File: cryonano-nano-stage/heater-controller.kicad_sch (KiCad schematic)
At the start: 13 parts, among them U3 1ED3141MU12FXUMA1

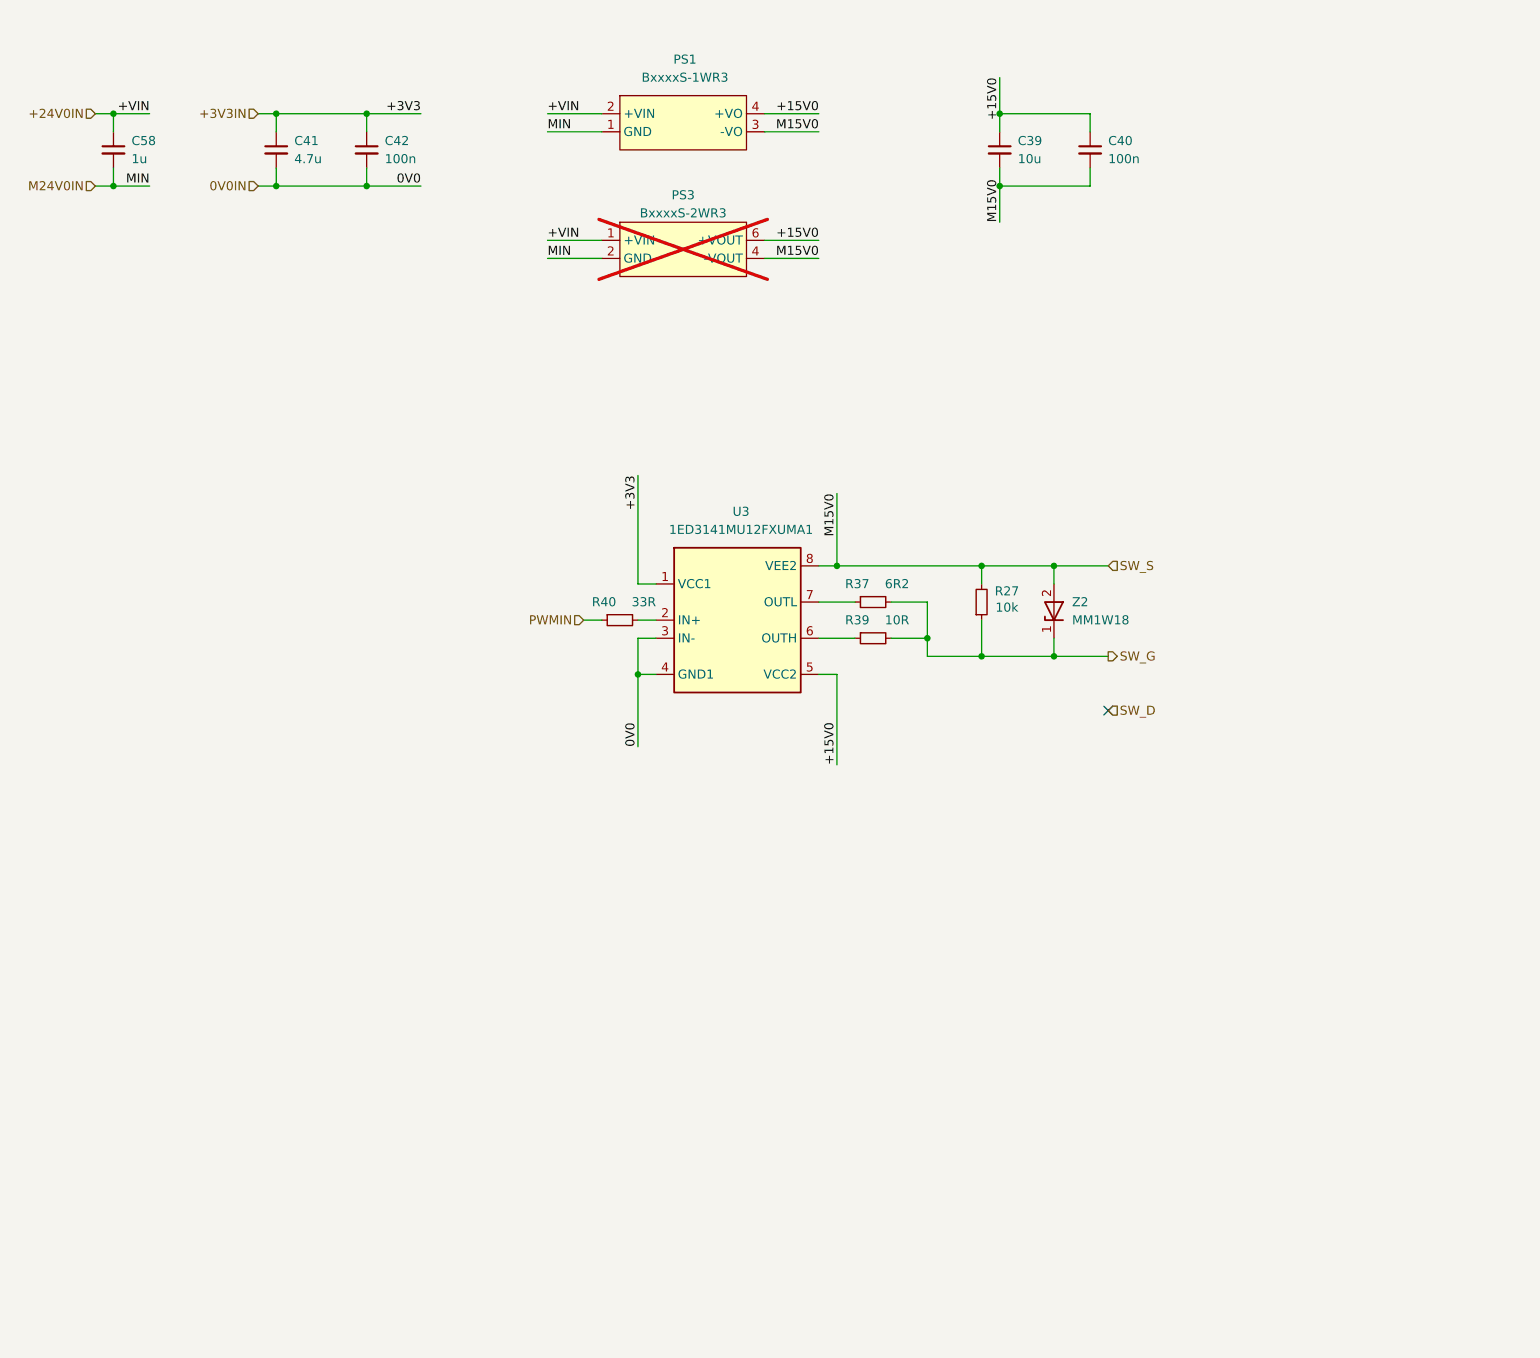
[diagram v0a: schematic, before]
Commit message: drc ok, review schematic
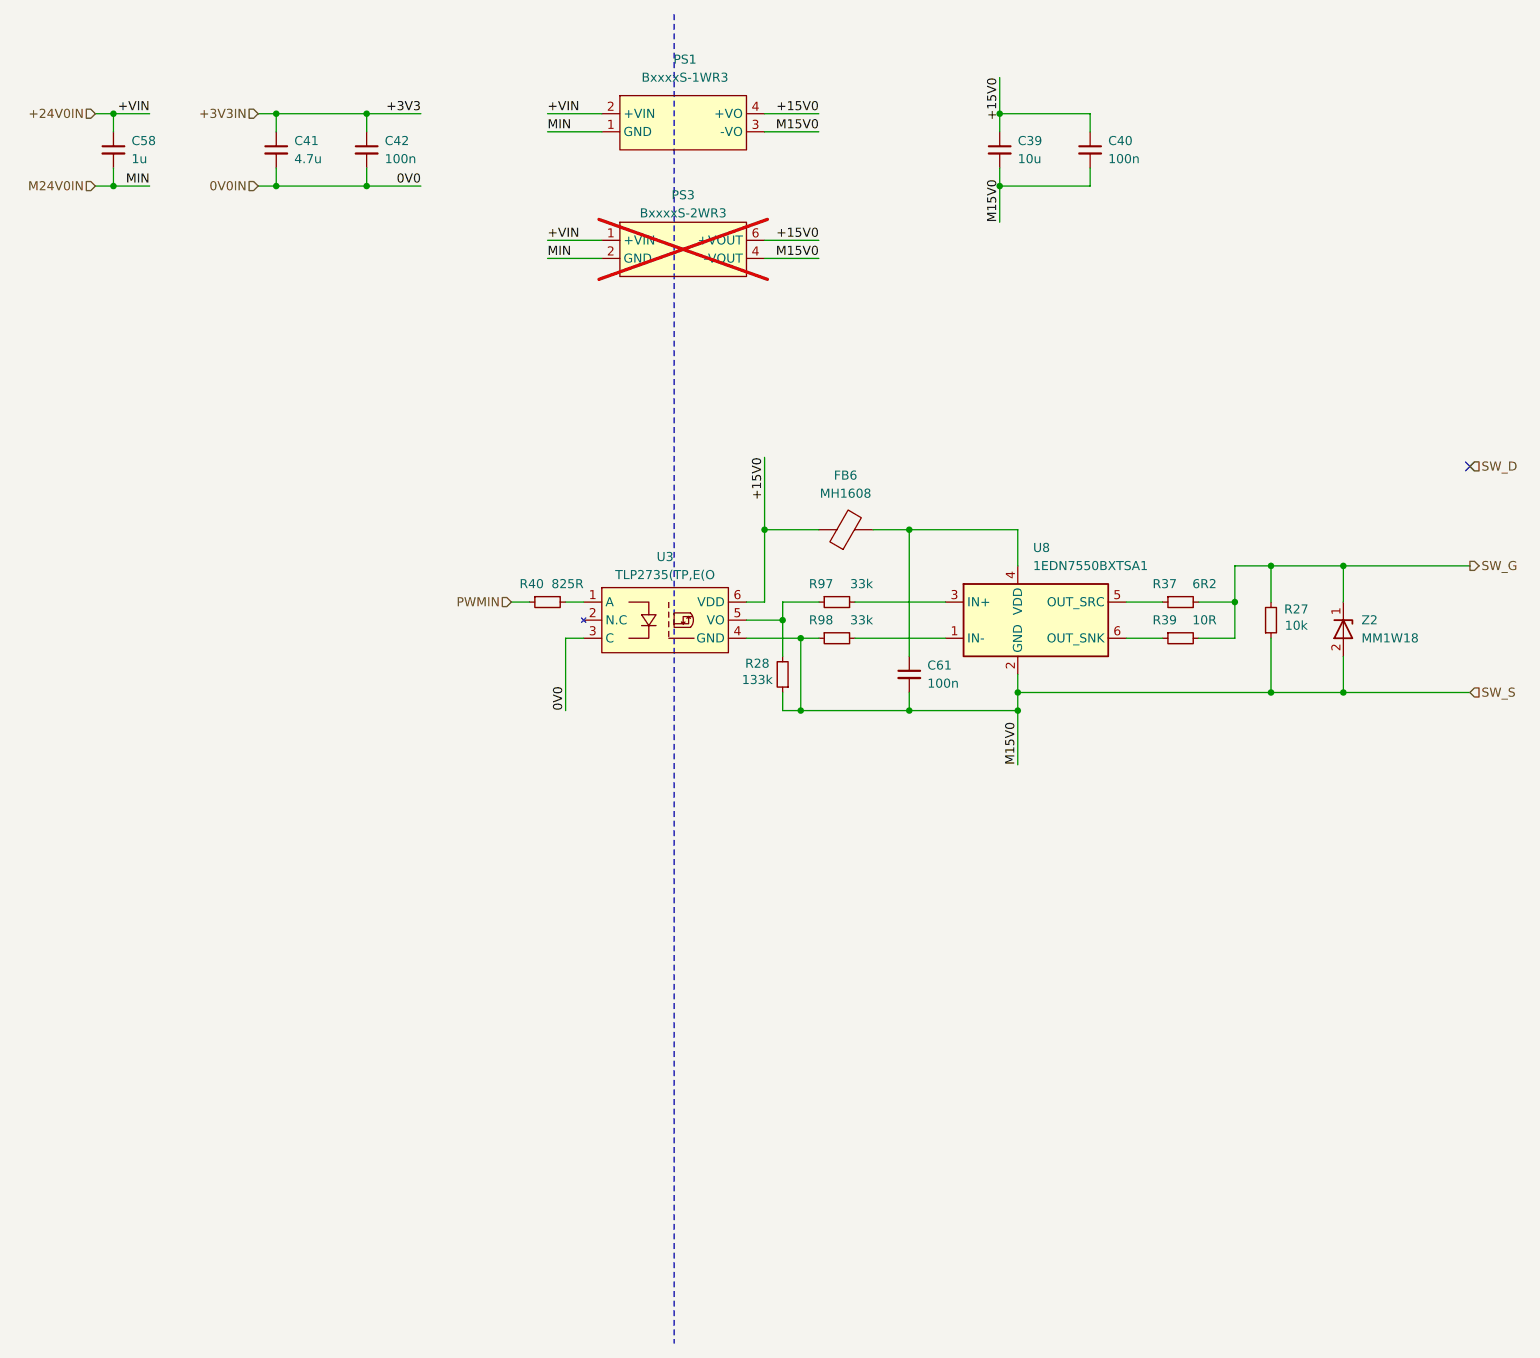
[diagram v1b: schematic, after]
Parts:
- removed U3: 1ED3141MU12FXUMA1, footprints:SOIC127P600X175-8N, symbol symbols:1ED3141MU12FXUMA1
- added C61: 100n, Capacitor_SMD:C_0603_1608Metric, symbol Device:C_Small
- added FB6: MH1608, Inductor_SMD:L_0603_1608Metric, symbol Device:FerriteBead
- added R28: 133k, Resistor_SMD:R_0603_1608Metric, symbol Device:R_Small
- added R97, R98: 33k, Resistor_SMD:R_0603_1608Metric, symbol Device:R_Small
- added U3: TLP2735(TP,E(O, footprints:SO-6L_10x3.84mm_P1.27mm, symbol symbols:TLP2735
- added U8: 1EDN7550BXTSA1, footprints:SOT95P280X145-6N, symbol symbols:1EDN7550BXTSA1
- C39: footprint Capacitor_SMD:C_1210_3225Metric -> Capacitor_SMD:C_0805_2012Metric; Manufacturer YAGEO -> (none); Order No. CC1210KFX7R9BB106 -> (none); Unit Price 10 31.1 -> (none)
- R40: value 33R -> 825R
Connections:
- net +15V0: now also FB6.1, U3.6 (VDD)
- net 0V0IN: now also U3.3 (C)
- net SW_G: now also R27.2; no longer R27.1
- net SW_S: now also R27.1, C61.2, R28.1, R98.1, U3.4 (GND), U8.2 (GND); no longer R27.2
- net at R39.1: now also U8.6 (OUT_SNK)
- net at R40.2: now also U3.1 (A)
- net at R37.1: now also U8.5 (OUT_SRC)
- new net: C61.1, FB6.2, U8.4 (VDD)
- new net: R98.2, U8.1 (IN-)
- new net: R28.2, R97.1, U3.5 (VO)
- new net: R97.2, U8.3 (IN+)
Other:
- moved on the sheet: R27, R37, R39, R40, Z2
